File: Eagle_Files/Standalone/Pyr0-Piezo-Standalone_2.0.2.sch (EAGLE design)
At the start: 71 parts, among them J1 FFC-15P-1MM, U1 ATMEGA48/88/168/328PA, U4 LM2902QT, X1 FFC-40P-0.5SH

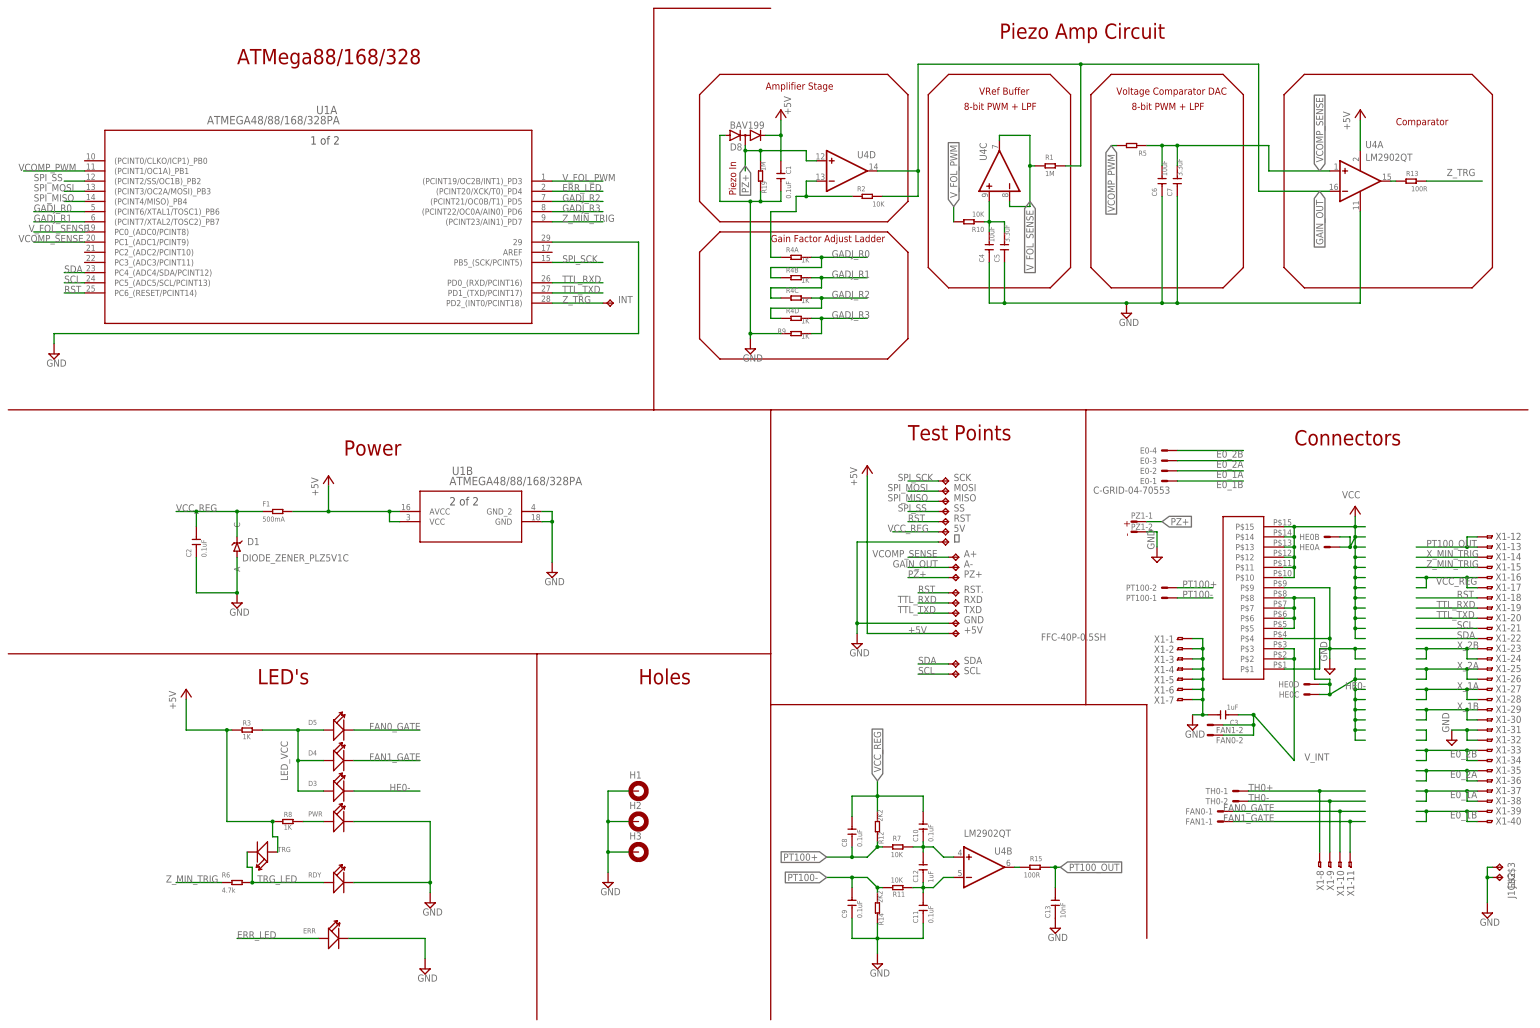
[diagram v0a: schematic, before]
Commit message: fixed some file encoding issues
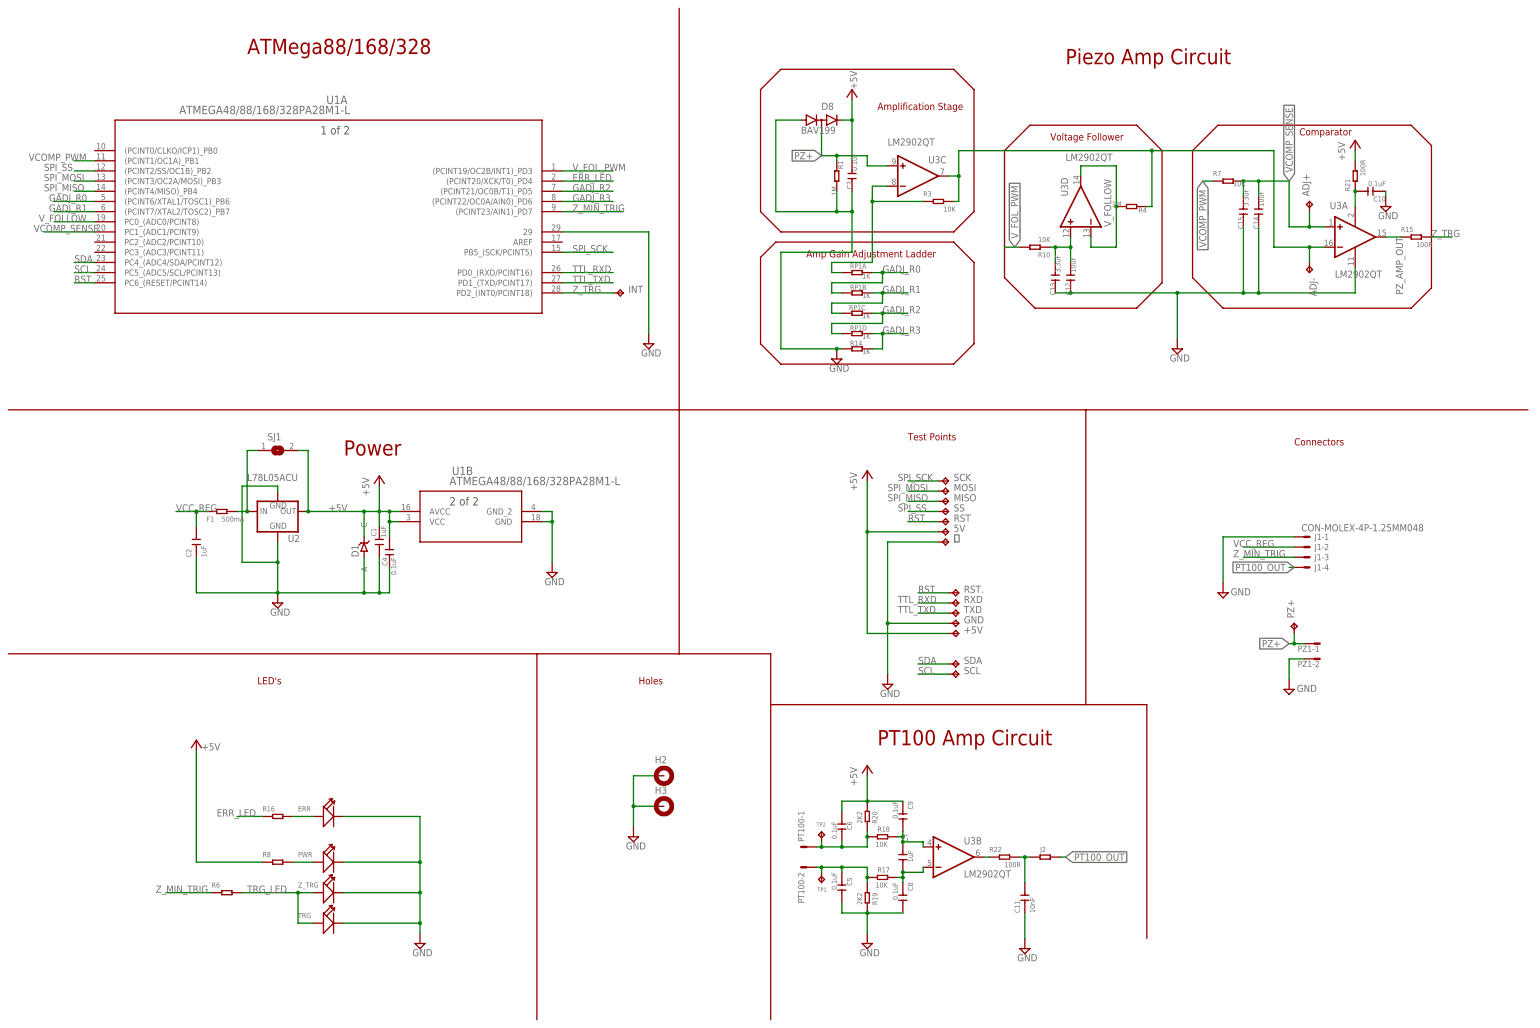
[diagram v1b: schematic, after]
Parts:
- removed A+, A-: TPTP13SQ, PiezoFFC:TPTP13SQ
- removed D3, D4, D5, RDY: (no value), PiezoFFC:SEEED-LED_SMD-LED-CLEAR-BLUE(0603)LED_0603
- removed E0: C-GRID-04-70553, PiezoFFC:C-GRID-04-70553
- removed FAN0, FAN1, TH0: CON-MOLEX-2P-1.27MM048, PiezoFFC:CON-MOLEX-2P-1.27MM048
- removed H1: HOLES_MOUNT-PAD-ROUND3.2, PiezoFFC:HOLES_MOUNT-PAD-ROUND3.2
- removed HE0: JST-2.54-2X2JST-DUPONT-2.54-2X2, PiezoFFC:JST-2.54-2X2JST-DUPONT-2.54-2X2
- removed R11, R2: 10K, PiezoFFC:SMD-RES-0R-5%-1/16W(0402)
- removed R12: 2K2, PiezoFFC:SMD-RES-0R-5%-1/16W(0402)
- removed R13: 100R, PiezoFFC:SMD-RES-0R-5%-1/16W(0402)
- removed R5: 10K, PiezoFFC:SEEED-RESISTOR_SMD-RES-1.5K-1%-1/10W(0603)DETAILED_MODEL
- removed R9: 1K, PiezoFFC:SMD-RES-0R-5%-1/16W(0402)
- removed U4: LM2902QT, PiezoFFC:LM2902QT
- removed X1: FFC-40P-0.5SH, PiezoFFC:FFC-40P-0.5SH
- added ADJ+, ADJ-: TPTP13SQ, PiezoFFC:TPTP13SQ
- added C14: 10uF, PiezoFFC:CERAMIC-1NF-50V-10%-X7R(0402)CAP_0402
- added C15: 3.3uF, PiezoFFC:CERAMIC-1NF-50V-10%-X7R(0402)CAP_0402
- added J2: (no value), PiezoFFC:SEEED-RESISTOR_SMD-RES-1.5K-1%-1/10W(0603)DETAILED_MODEL
- added R16: (no value), PiezoFFC:SMD-RES-0R-5%-1/16W(0402)
- added R17, R18: 10K, PiezoFFC:SMD-RES-0R-5%-1/16W(0402)
- added R20: 2K2, PiezoFFC:SMD-RES-0R-5%-1/16W(0402)
- added R21, R22: 100R, PiezoFFC:SMD-RES-0R-5%-1/16W(0402)
- added RP1: 1K, PiezoFFC:RESISTOR_NETWORK_X40804_L
- added SJ1: (no value), PiezoFFC:SJM
- added TP1, TP2: TPTP09R, PiezoFFC:TPTP09R
- added U2: L78L05ACU, PiezoFFC:L78L05ACU
- added U3: LM2902QT, PiezoFFC:LM2902QT
- added Z_TRG: (no value), PiezoFFC:SEEED-LED_SMD-LED-CLEAR-BLUE(0603)LED_0603
- C1, C2: value 0.1uF -> 1uF; device PiezoFFC:CERAMIC-1NF-50V-10%-X7R(0402)CAP_0402 -> PiezoFFC:SEEED-CAPACITOR_CERAMIC-10UF-25V-10%-X5R(0805)CAP_0603_GEN
- C11: value 0.1uF -> 10nF
- C12: value 1uF -> 10uF
- C13: value 10nF -> 3.3uF
- C3: value 1uF -> 0.1uF; device PiezoFFC:SEEED-CAPACITOR_CERAMIC-10UF-25V-10%-X5R(0805)CAP_0603_GEN -> PiezoFFC:CERAMIC-1NF-50V-10%-X7R(0402)CAP_0402
- C4, C6: value 10uF -> 0.1uF
- C5: value 3.3uF -> 0.1uF; device PiezoFFC:SEEED-CAPACITOR_CERAMIC-10UF-25V-10%-X5R(0805)CAP_0603_GEN -> PiezoFFC:CERAMIC-1NF-50V-10%-X7R(0402)CAP_0402
- C7: value 3.3uF -> 1uF; device PiezoFFC:SEEED-CAPACITOR_CERAMIC-10UF-25V-10%-X5R(0805)CAP_0603_GEN -> PiezoFFC:CERAMIC-1NF-50V-10%-X7R(0402)CAP_0402
- D1: value DIODE_ZENER_PLZ5V1C -> ZENER_DIODE_PLZ5V1C; device PiezoFFC:DIODE_ZENER_PLZ5V1C -> PiezoFFC:ZENER_DIODE_PLZ5V1C
- F1: device PiezoFFC:SEEED-RESISTOR_SMD-RES-1.5K-1%-1/10W(0603)DETAILED_MODEL -> PiezoFFC:SMD-RES-0R-5%-1/16W(0402)
- H2, H3: value HOLES_MOUNT-PAD-ROUND3.2 -> HOLES_MOUNT-PAD-ROUND2.8; device PiezoFFC:HOLES_MOUNT-PAD-ROUND3.2 -> PiezoFFC:HOLES_MOUNT-PAD-ROUND2.8
- J1: value FFC-15P-1MM -> CON-MOLEX-4P-1.25MM048; device PiezoFFC:FFC-15P-1MM -> PiezoFFC:CON-MOLEX-4P-1.25MM048
- R14: value 2K2 -> 1K
- R19: value 1M -> 2K2
- R3: value 1K -> 10K
- R4: value 1K -> 1M; device PiezoFFC:RESISTOR_NETWORK_X40804 -> PiezoFFC:SMD-RES-0R-5%-1/16W(0402)
- R6: value 4.7k -> (none)
- R8: value 1K -> (none)
- U1: value ATMEGA48/88/168/328PA -> ATMEGA48/88/168/328PA28M1-L; device PiezoFFC:ATMEGA48/88/168/328PA -> PiezoFFC:ATMEGA48/88/168/328PA28M1-L
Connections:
- net N$2 renamed PWR_LED
- removed net E0_1A: E0-2.S, X1-37.1, X1-38.1
- removed net E0_1B: E0-1.S, X1-39.1, X1-40.1
- removed net E0_2A: E0-3.S, X1-35.1, X1-36.1
- removed net E0_2B: E0-4.S, X1-33.1, X1-34.1
- removed net FAN0_GATE: D5.-, FAN0-1.S, X1-10.1
- removed net FAN1_GATE: D4.-, FAN1-1.S, X1-11.1
- removed net GAIN_FB: R2.1, R4A.1, U4D.-IN
- removed net HE0-: D3.-, HE0C.S, HE0D.S, J1G$1.P$5, J1G$1.P$6, J1G$1.P$7, J1G$1.P$8
- removed net LED_VCC: D3.+, D4.+, D5.+, R3.2
- removed net PT100+: C8.1, PT100-2.S, R12.1, R7.2
- removed net PT100-: C9.2, PT100-1.S, R11.2, R14.2
- removed net PT100_AMP+: C10.1, C12.2, R7.1, U4B.+IN
- removed net PT100_AMP-: C11.2, C12.1, R11.1, U4B.-IN
- removed net PT100_R: R15.2, U4B.OUT
- removed net TH0+: TH0-1.S, X1-8.1
- removed net TH0-: TH0-2.S, X1-9.1
- removed net VCC: HE0A.S, HE0B.S, J1G$1.P$10, J1G$1.P$11, J1G$1.P$12, J1G$1.P$13, J1G$1.P$14, J1G$1.P$15
- removed net VREF_IN: C4.2, C5.2, R10.1, U4C.+IN
- removed net V_FOL_SENSE: R1.1, U1A.PC0_(ADC0/PCINT8), U4C.-IN, U4C.OUT
- removed net V_INT: C3.1, FAN0-2.S, FAN1-2.S, J1G$1.P$2, J1G$1.P$3
- removed net X_1A: X1-27.1, X1-28.1
- removed net X_1B: X1-29.1, X1-30.1
- removed net X_2A: X1-25.1, X1-26.1
- removed net X_2B: X1-23.1, X1-24.1
- removed net X_MIN_TRIG: X1-14.1
- new net AMP_VCC: C10.2, R21.1, U3P.V+
- new net ERR_LED)R: ERR.+, R16.2
- new net GAIN_ADJ: R3.1, RP1A.1, U3C.-IN
- new net PT100_JUMP: C11.2, J2.1, R22.2
- new net PTAMP+: C7.2, C9.2, R18.2, U3B.+IN
- new net PTAMP-: C7.1, C8.1, R17.2, U3B.-IN
- new net PT_AMP: R22.1, U3B.OUT
- new net PT_IN+: C6.2, PT100-1.S, R18.1, R20.2, TP2.TP
- new net PT_IN-: C5.1, PT100-2.S, R17.1, R19.1, TP1.TP
- new net VCC_FUSE: F1.2, SJ1.1, U2.IN
- new net V_FOLLOW: R4.2, U1A.PC0_(ADC0/PCINT8), U3D.-IN, U3D.OUT
- new net V_FOL_ADJ: C12.2, C13.2, R10.1, U3D.+IN
- net +5V: now also 5V.TP, C1.2, C3.2, C4.2, C6.1, C9.1, D1.C, R20.1, R21.2, SJ1.2, U2.OUT; no longer C1.1, F1.2, R3.1, TRG.+, U4P.V+
- net ERR_LED: now also R16.1; no longer ERR.+
- net GADJ_R0: now also RP1A.2, RP1B.1; no longer R4A.2, R4B.1
- net GADJ_R1: now also RP1B.2, RP1C.1; no longer R4B.2, R4C.1
- net GADJ_R2: now also RP1C.2, RP1D.1; no longer R4C.2, R4D.1
- net GADJ_R3: now also R14.2, RP1D.2; no longer R4D.2, R9.2
- net GAIN_OUT: now also ADJ-.TP, R3.2, R4.1, U3A.-IN, U3C.OUT; no longer A-.TP, R1.2, R2.2, U4A.-IN, U4D.OUT
- net GND: now also C1.1, C10.1, C12.1, C14.1, C15.1, C3.1, C5.2, C8.2, J1-1.S, R1.2, R19.2, TRG.-, U2.GND, U2.PAD, U3P.V-, Z_TRG.-; no longer C1.2, C3.2, C5.1, C6.1, C7.1, C9.1, H1.MOUNT, J1G$1.P$1, J1G$1.P$4, J1G$1.P$9, J1G$2.TP, J1G$3.TP, R19.1, R9.1, RDY.-, U4P.V-, X1-1.1, X1-2.1, X1-3.1, X1-31.1, X1-32.1, X1-4.1, X1-5.1, X1-6.1, X1-7.1
- net PT100_OUT: now also J1-4.S, J2.2; no longer C13.2, R15.1, X1-12.1, X1-13.1
- net PZ+: now also R1.1, U3C.+IN; no longer R19.2, U4D.+IN
- net PZ_AMP_OUT: now also R15.1, U3A.OUT; no longer R13.1, U4A.OUT
- net RST: no longer X1-18.1
- net SCL: no longer X1-21.1
- net SDA: no longer X1-22.1
- net TRG_LED: now also TRG.+, Z_TRG.+; no longer RDY.+, TRG.-
- net TTL_RXD: no longer X1-19.1
- net TTL_TXD: no longer X1-20.1
- net VCC_REG: now also J1-2.S; no longer 5V.TP, C10.2, C8.2, D1.C, R12.2, X1-16.1, X1-17.1
- net VCOMP_PWM: now also R7.1; no longer R5.2
- net VCOMP_SENSE: now also ADJ+.TP, C14.2, C15.2, R7.2, U3A.+IN; no longer A+.TP, C6.2, C7.2, R5.1, U4A.+IN
- net Z_MIN_TRIG: now also J1-3.S; no longer X1-15.1
- net Z_TRG: now also R15.2; no longer R13.2
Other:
- note added: "Amp Gain Adjustment Ladder"
- note added: "Amplification Stage"
- note added: "PT100 Amp Circuit"
- note added: "Voltage Follower"
- note removed: "- +"
- note removed: "8-bit PWM + LPF"
- note removed: "Amplifier Stage"
- note removed: "Gain Factor Adjust Ladder"
- note removed: "Piezo In"
- note removed: "VRef Buffer"
- note removed: "Voltage Comparator DAC"
- moved on the sheet: C1, C10, C11, C12, C13, C3, C4, C5, C6, C7, C8, C9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
